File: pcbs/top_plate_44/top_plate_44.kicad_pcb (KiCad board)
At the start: 2 copper layers, 147.4 x 108 mm, 6 parts

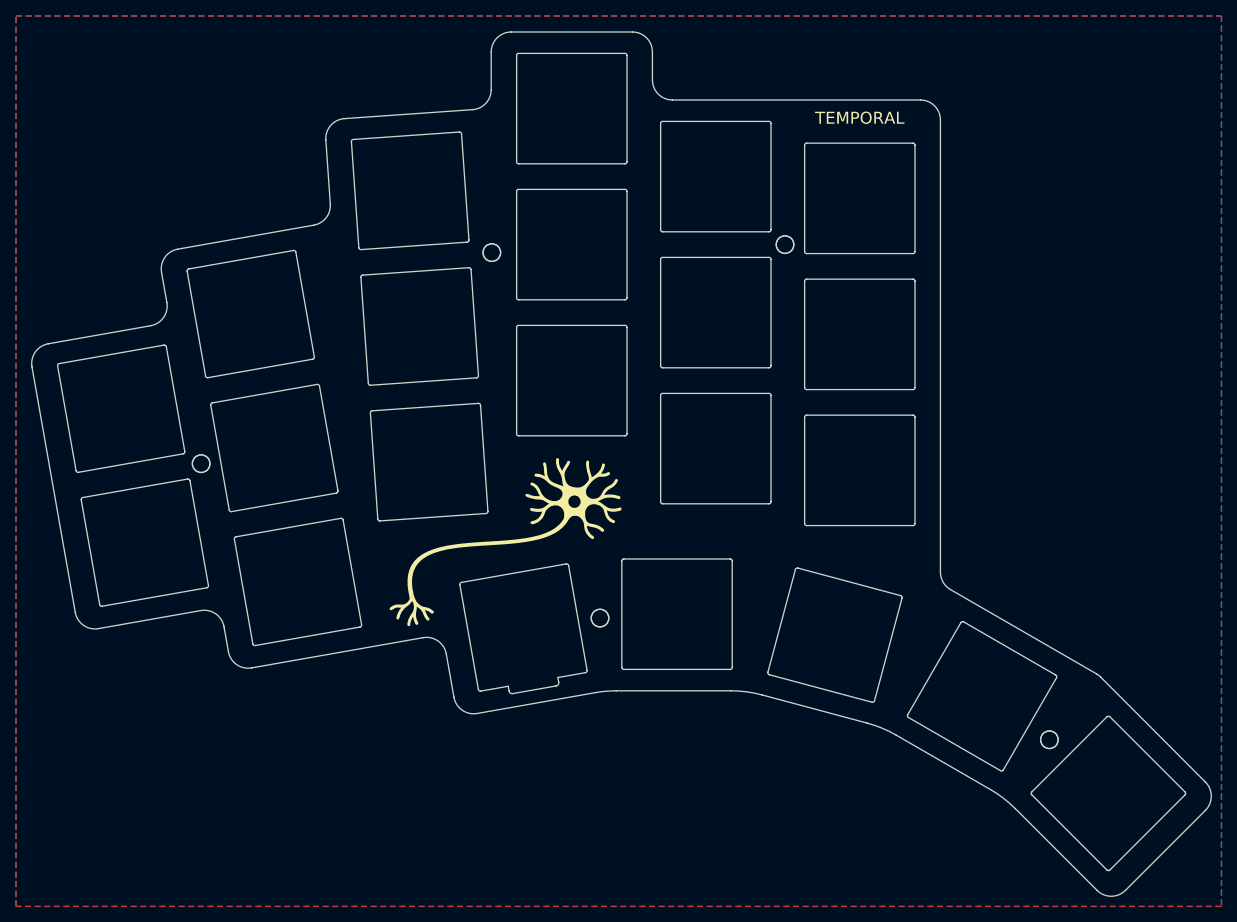
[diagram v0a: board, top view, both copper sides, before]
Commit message: update naming and gen files
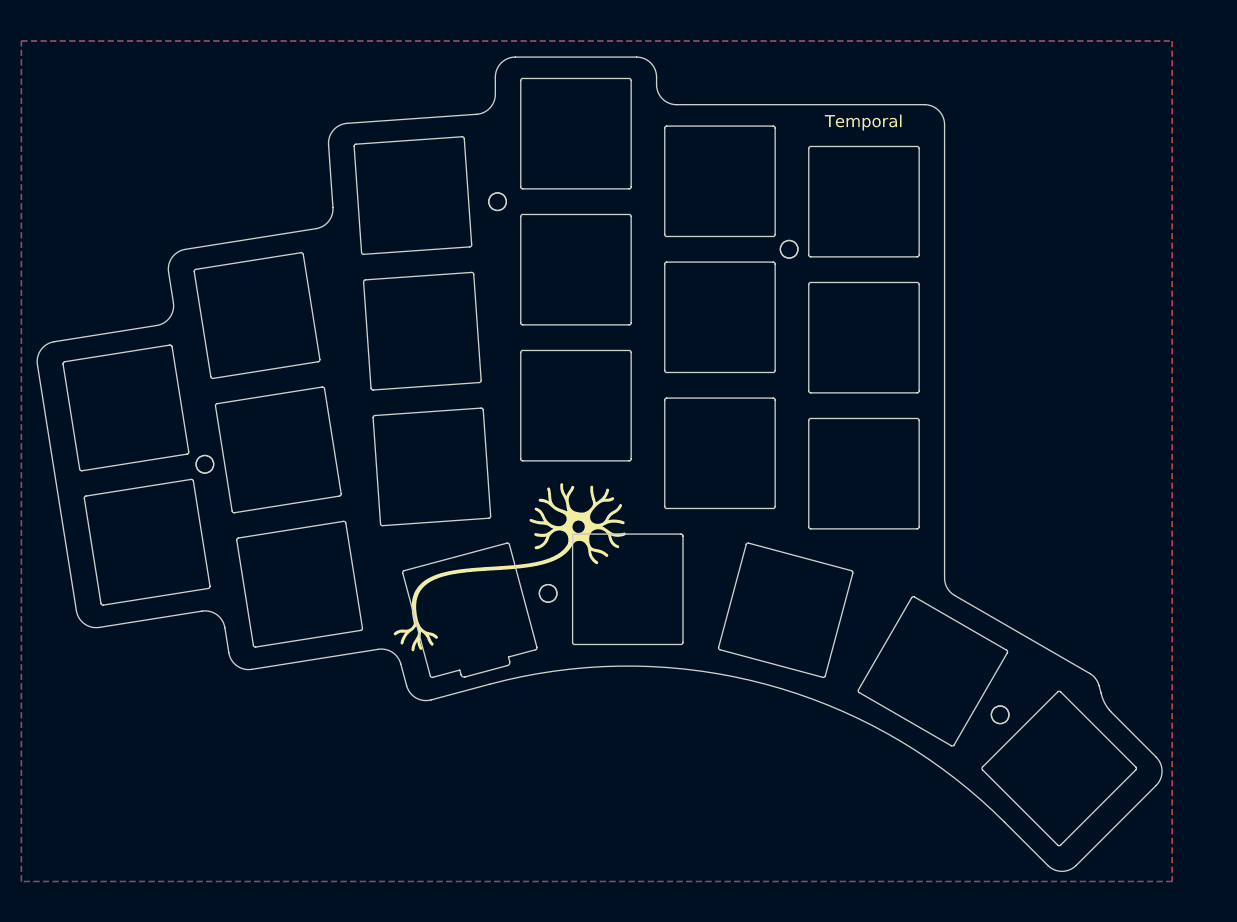
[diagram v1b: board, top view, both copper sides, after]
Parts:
- moved MH4 7.18 mm to (97.5, 89.6), turned to 15 degrees
- moved MH3 6.90 mm to (154.0, 104.8)
- moved MH1 6.41 mm to (91.1, 40.6)
- moved G1 3.18 mm to (92.7, 86.3)
- moved MH2 0.78 mm to (127.6, 46.6)
- moved MH5 0.47 mm to (54.6, 73.5), turned to 9 degrees
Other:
- board size 147.4 x 108 mm -> 140.6 x 101.8 mm
- board text added: "Temporal"
- board text removed: "TEMPORAL"
